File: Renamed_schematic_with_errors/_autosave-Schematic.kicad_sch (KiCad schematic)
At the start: 23 parts, among them J1 STEP/DIR, J2 VCC_IO, J3 MISC, P9 VM

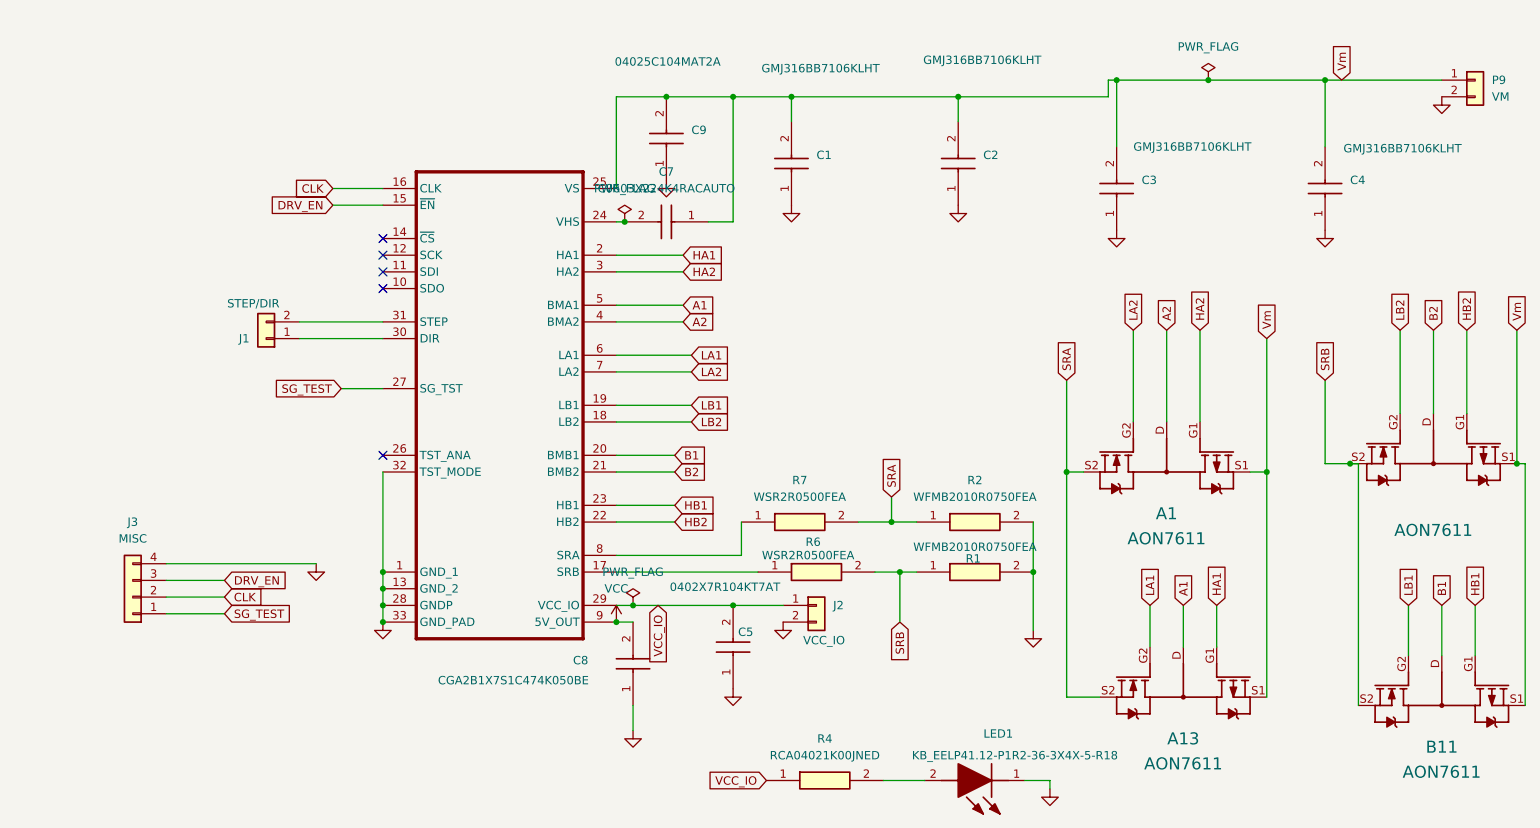
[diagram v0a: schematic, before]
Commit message: this is alot
good luck
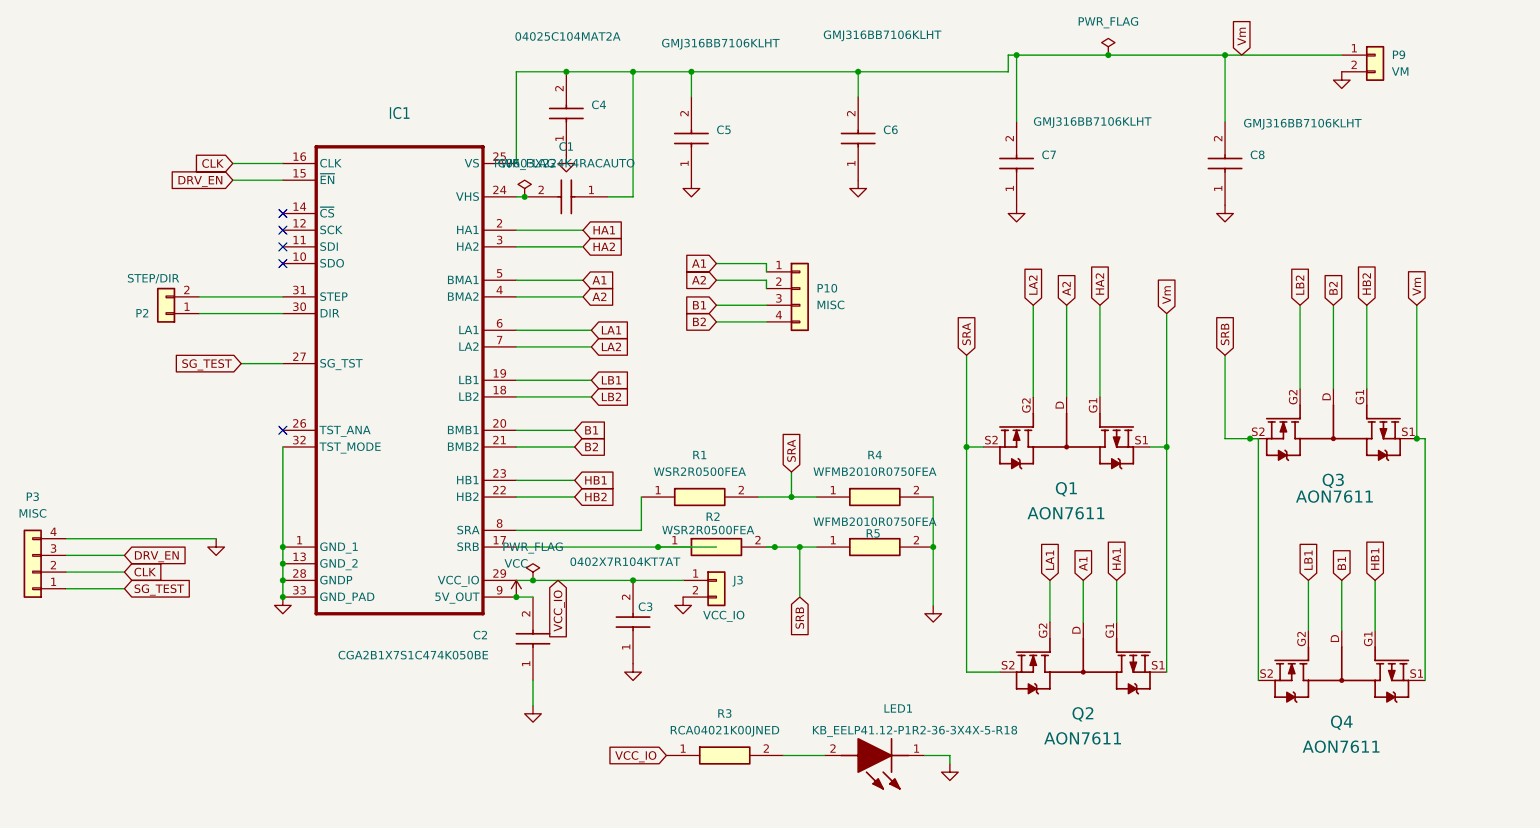
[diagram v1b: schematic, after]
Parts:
- removed A1, A13, B1, B11: AON7611, AON7611, symbol TMC262_BOB40_V1_2:AON7611
- removed C1, C2, C3, C4: GMJ316BB7106KLHT, CAPPC3216X125N, symbol GMJ316BB7106KLHT:GMJ316BB7106KLHT
- removed C5: 0402X7R104KT7AT, CAPC1005X61N, symbol 0402X7R104KT7AT:0402X7R104KT7AT
- removed C7: C0603X224K4RACAUTO, C0603, symbol C0603X224K4RACAUTO:C0603X224K4RACAUTO
- removed C8: CGA2B1X7S1C474K050BE, CAPC1005X55N, symbol CGA2B1X7S1C474K050BE:CGA2B1X7S1C474K050BE
- removed C9: 04025C104MAT2A, CAPC1005X56N, symbol 04025C104MAT2A:04025C104MAT2A
- removed J1: STEP/DIR, symbol Connector_Generic:Conn_01x02
- removed J2: VCC_IO, symbol Connector_Generic:Conn_01x02
- removed J3: MISC, symbol Connector_Generic:Conn_01x04
- removed R1, R2: WFMB2010R0750FEA, RESC5125X65N, symbol WFMB2010R0750FEA:WFMB2010R0750FEA
- removed R4: RCA04021K00JNED, RESC1005X40N, symbol RCA04021K00JNED:RCA04021K00JNED
- removed R6, R7: WSR2R0500FEA, RESM11670X254N, symbol WSR2R0500FEA:WSR2R0500FEA
- added C1: C0603X224K4RACAUTO, Capacitor_SMD:C_0603_1608Metric, symbol C0603X224K4RACAUTO:C0603X224K4RACAUTO
- added C2: CGA2B1X7S1C474K050BE, Capacitor_SMD:C_0402_1005Metric, symbol CGA2B1X7S1C474K050BE:CGA2B1X7S1C474K050BE
- added C3: 0402X7R104KT7AT, Capacitor_SMD:C_0402_1005Metric, symbol 0402X7R104KT7AT:0402X7R104KT7AT
- added C4: 04025C104MAT2A, Capacitor_SMD:C_0402_1005Metric, symbol 04025C104MAT2A:04025C104MAT2A
- added C5, C6, C7, C8: GMJ316BB7106KLHT, Capacitor_SMD:C_1206_3216Metric, symbol GMJ316BB7106KLHT:GMJ316BB7106KLHT
- added J3: VCC_IO, Connector_PinHeader_2.54mm:PinHeader_1x02_P2.54mm_Vertical, symbol Connector_Generic:Conn_01x02
- added P10: MISC, Connector_Phoenix_MSTB:PhoenixContact_MSTBA_2,5_4-G_1x04_P5.00mm_Horizontal, symbol Connector_Generic:Conn_01x04
- added P2: STEP/DIR, Connector_PinHeader_2.54mm:PinHeader_1x02_P2.54mm_Vertical, symbol Connector_Generic:Conn_01x02
- added P3: MISC, Connector_PinHeader_2.54mm:PinHeader_1x04_P2.54mm_Vertical, symbol Connector_Generic:Conn_01x04
- added Q1, Q2, Q3, Q4: AON7611, Package_SO:SOIC-8_3.9x4.9mm_P1.27mm, symbol TMC262_BOB40_V1_2:AON7611
- added R1, R2: WSR2R0500FEA, Resistor_SMD:R_Shunt_Vishay_WSR2_WSR3, symbol WSR2R0500FEA:WSR2R0500FEA
- added R3: RCA04021K00JNED, Resistor_SMD:R_0402_1005Metric, symbol RCA04021K00JNED:RCA04021K00JNED
- added R4, R5: WFMB2010R0750FEA, Resistor_SMD:R_2010_5025Metric, symbol WFMB2010R0750FEA:WFMB2010R0750FEA
- IC1: footprint TMC262-LA:TMC_QFN32_0.5_5.0X5.0 -> Package_DFN_QFN:QFN-32-1EP_5x5mm_P0.5mm_EP3.3x3.3mm_ThermalVias
- LED1: footprint KBEELP4112P1R2363X4X5R18 -> LED_SMD:LED_0805_2012Metric
- P9: footprint (none) -> Connector_Phoenix_MSTB:PhoenixContact_MSTBA_2,5_2-G_1x02_P5.00mm_Horizontal
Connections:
- net A1: now also P10.1 (Pin_1), Q2.D
- net A2: now also P10.2 (Pin_2), Q1.D
- net B1: now also P10.3 (Pin_3), Q4.D
- net B2: now also P10.4 (Pin_4), Q3.D
- net CLK: now also P3.2 (Pin_2)
- net DRV_EN: now also P3.3 (Pin_3)
- net GND: now also C2.1, C3.1, C4.1, C5.1, C6.1, C7.1, C8.1, J3.2 (Pin_2), P3.4 (Pin_4), R4.2, R5.2
- net HA1: now also Q2.G1
- net HA2: now also Q1.G1
- net HB1: now also Q4.G1
- net HB2: now also Q3.G1
- net LA1: now also Q2.G2
- net LA2: now also Q1.G2
- net LB1: now also Q4.G2
- net LB2: now also Q3.G2
- net SG_TEST: now also P3.1 (Pin_1)
- net SRA: now also Q1.S2, Q2.S2, R1.2, R4.1
- net SRB: now also Q3.S2, Q4.S2, R2.2, R5.1
- net VCC: now also C2.2
- net VCC_IO: now also C3.2, J3.1 (Pin_1), R3.1
- net Vm: now also C1.1, C4.2, C5.2, C6.2, C7.2, C8.2, Q1.S1, Q2.S1, Q3.S1, Q4.S1
- net at IC1.24 (VHS): now also C1.2
- net at IC1.8 (SRA): now also R1.1
- net at IC1.17 (SRB): now also R2.1
- net at IC1.30 (DIR): now also P2.1 (Pin_1)
- net at IC1.31 (STEP): now also P2.2 (Pin_2)
- net at LED1.2 (A): now also R3.2
